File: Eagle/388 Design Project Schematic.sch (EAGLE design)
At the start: 32 parts, among them IC1 MC33269ST-3.3T3, T1 2N2222, T2 2N2222, U1 328P, X10 332-02, X4 Screw Hole 1, X9 332-02

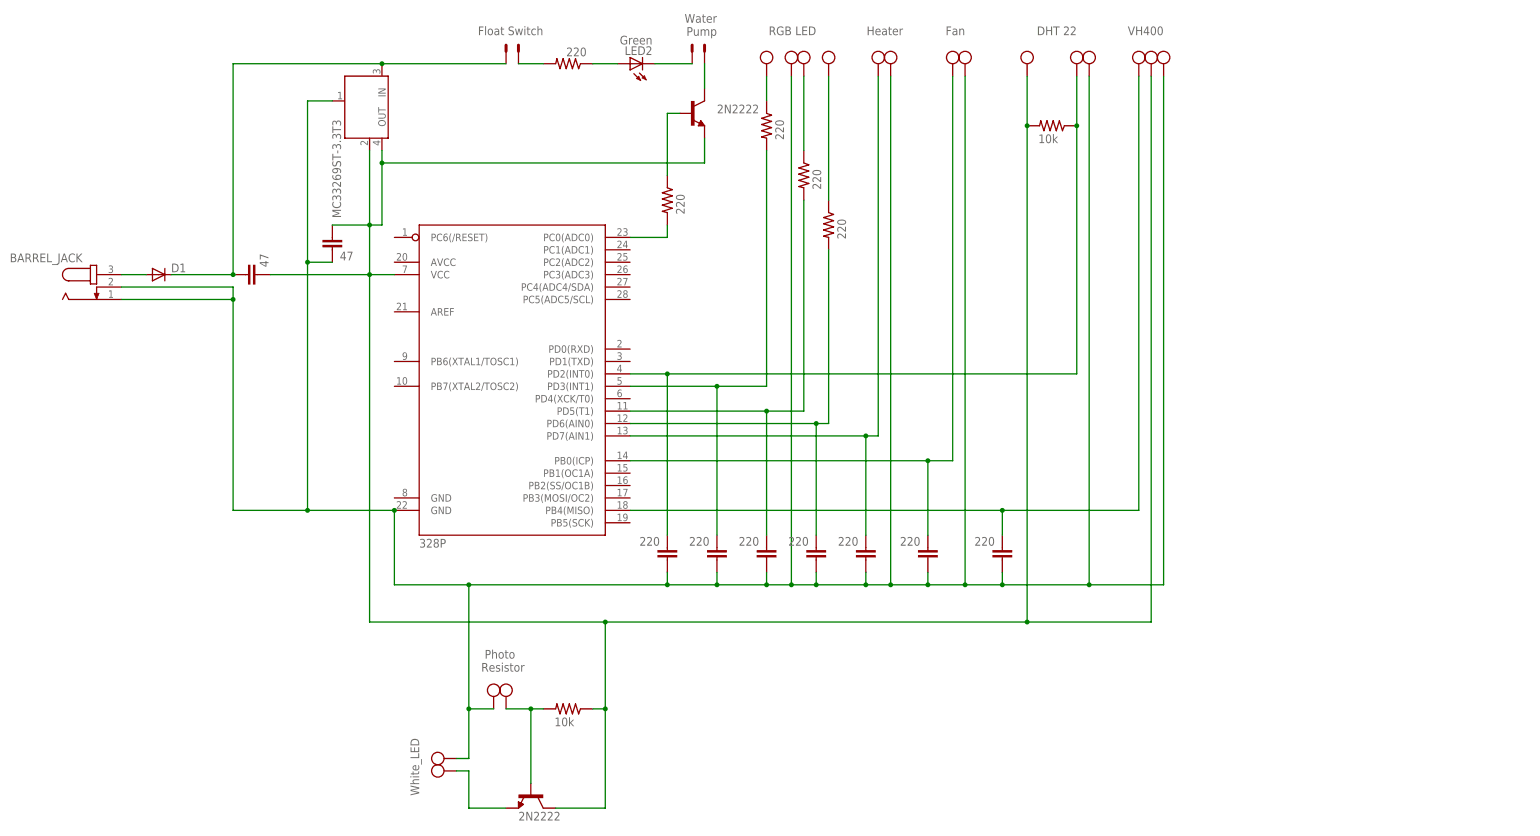
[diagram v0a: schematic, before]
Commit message: Add files via upload
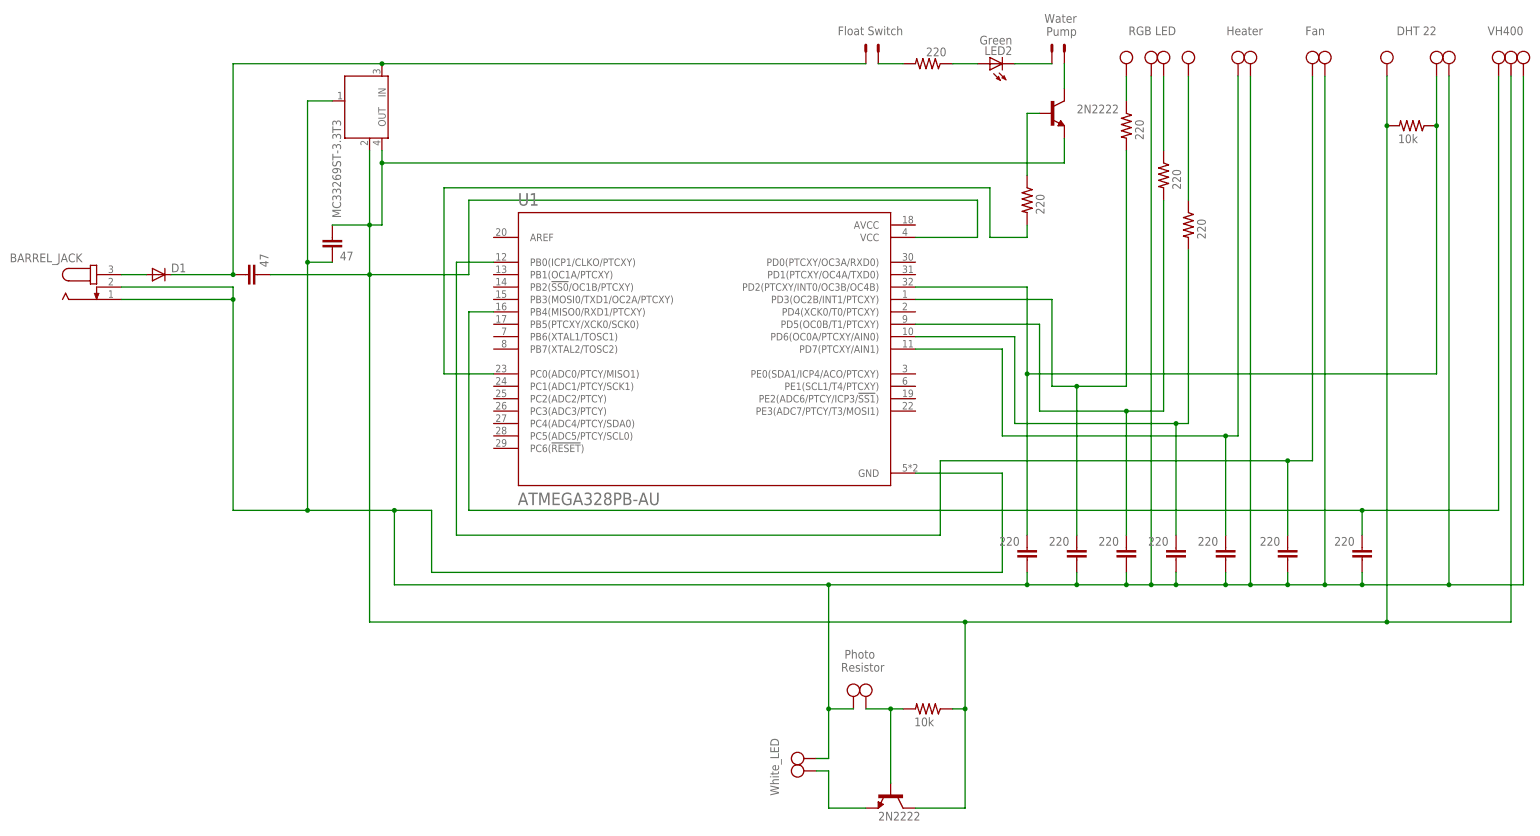
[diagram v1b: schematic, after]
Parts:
- removed X3: (no value), con-ptr500:AK300/2
- added X5: (no value), con-ptr500:AK300/3
- added X8: (no value), ECE388:1X02_5MM_SCREW
- U1: value 328P -> ATMEGA328PB-AU; device SparkFun-IC-Microcontroller:ATMEGA328P_PDIP -> ATMEGA328PB-AU:ATMEGA328PB-AU
- X1: device con-ptr500:AK300/2 -> ECE388:1X02_5MM_SCREW
- X4: value Screw Hole 1 -> (none); device con-phoenix-smkdsp:SMKDSP_1,5/4 -> ECE388:1X02_5MM_SCREW
- X6: device con-wago-500:W237-103 -> con-ptr500:AK300/4
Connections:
- net N$10: now also U1.PB0(ICP1/CLKO/PTCXY), X8-2.KL; no longer U1.PB0(ICP), X3-1.KL
- net N$12: now also U1.PD6(OC0A/PTCXY/AIN0); no longer U1.PD6(AIN0)
- net N$13: now also U1.PD5(OC0B/T1/PTCXY); no longer U1.PD5(T1)
- net N$14: now also X6-2.KL; no longer X4-3.KL
- net N$15: now also X6-1.KL; no longer X4-4.KL
- net N$2: now also X6-4.KL; no longer X4-1.KL
- net N$25: now also U1.PD2(PTCXY/INT0/OC3B/OC4B), X1-1.KL; no longer U1.PD2(INT0), X6-2.KL
- net N$26: now also U1.PD7(PTCXY/AIN1), X4-2.KL; no longer U1.PD7(AIN1), X1-1.KL
- net N$5: now also U1.PC0(ADC0/PTCY/MISO1); no longer U1.PC0(ADC0)
- net N$6: now also U1.GND, X4-1.KL, X6-3.KL, X8-1.KL; no longer U1.GND@2, X3-2.KL, X4-2.KL, X6-1.KL
- net N$7: now also X5-3.KL; no longer X6-3.KL
- net N$8: now also U1.PB4(MISO0/RXD1/PTCXY); no longer U1.PB4(MISO)
- net N$9: now also U1.PD3(OC2B/INT1/PTCXY); no longer U1.PD3(INT1)
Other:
- moved on the sheet: LED2
